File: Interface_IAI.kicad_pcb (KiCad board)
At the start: 2 copper layers, 54 x 63 mm, 20 parts, among them J1 ADWIN_DIO32, J2 ALIM_5V, J3 SCON_PULSE, J4 SCON_FEEDBACK, J5 ADWIN_CO4T, U1 AM26LS31CN, U2 AM26LS32ACN

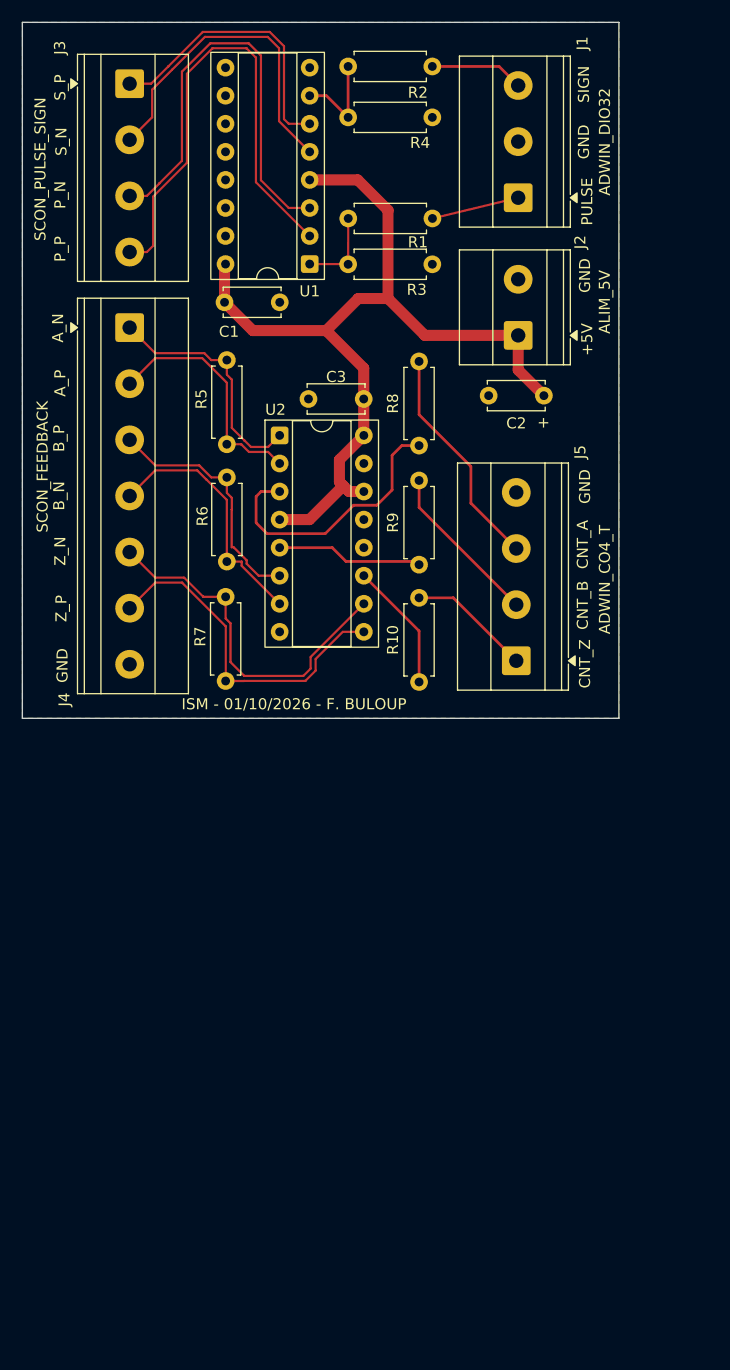
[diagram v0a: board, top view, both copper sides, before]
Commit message: Update board
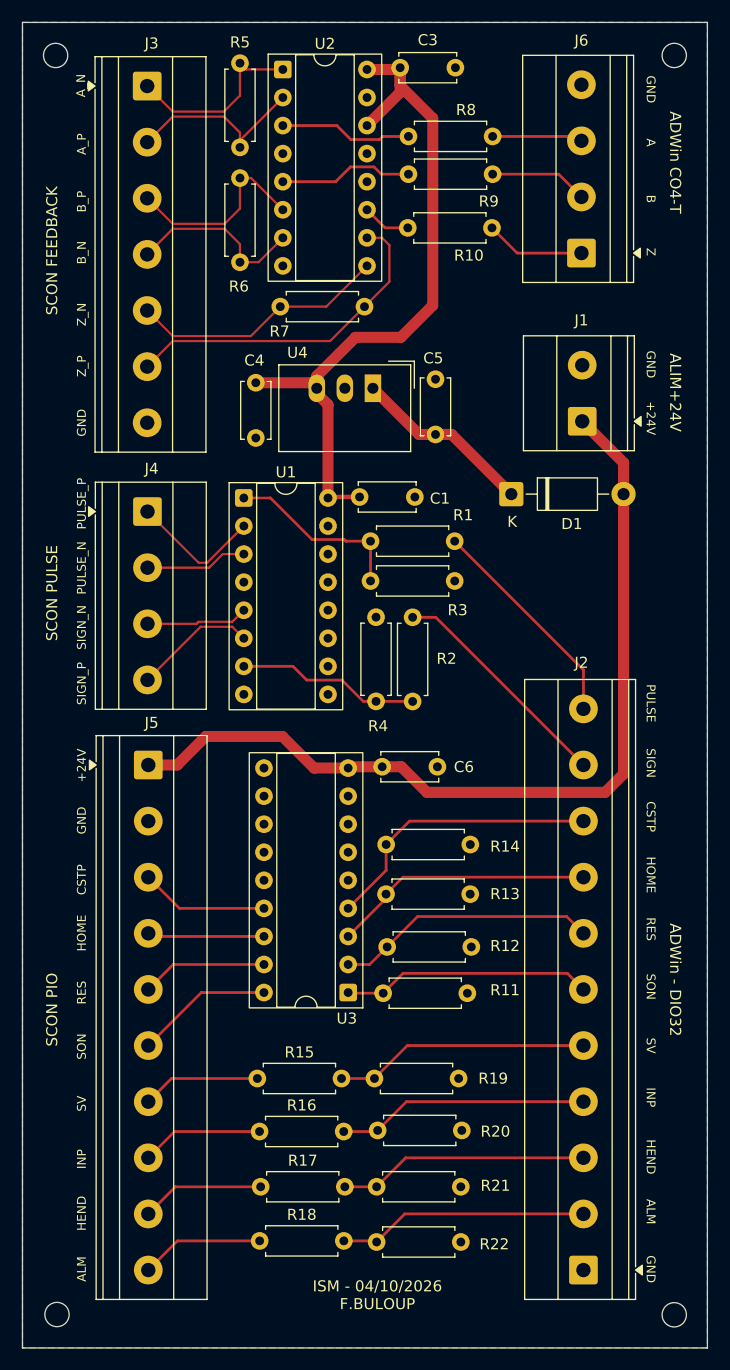
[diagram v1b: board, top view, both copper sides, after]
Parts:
- removed C2: 10uF, Capacitor_THT:C_Disc_D5.0mm_W2.5mm_P5.00mm
- added C4: 10uF, Capacitor_THT:C_Disc_D5.0mm_W2.5mm_P5.00mm, F.Cu at (71.1, 82.6)
- added C5: 10uF 50V, Capacitor_THT:C_Disc_D5.0mm_W2.5mm_P5.00mm, F.Cu at (87.4, 87.3)
- added C6: 100nF, Capacitor_THT:C_Disc_D5.0mm_W2.5mm_P5.00mm, F.Cu at (82.6, 117.4)
- added D1: 1N5819, Diode_THT:D_DO-41_SOD81_P10.16mm_Horizontal, F.Cu at (94.3, 92.7)
- added H1: MountingHole, MountingHole:MountingHole_2.2mm_M2, F.Cu at (109.0, 53.0)
- added H2: MountingHole, MountingHole:MountingHole_2.2mm_M2, F.Cu at (109.0, 167.0)
- added H3: MountingHole, MountingHole:MountingHole_2.2mm_M2, F.Cu at (53.0, 53.0)
- added H4: MountingHole, MountingHole:MountingHole_2.2mm_M2, F.Cu at (53.1, 167.0)
- added J6: ADWin CO4-T, TerminalBlock_Phoenix:TerminalBlock_Phoenix_MKDS-1,5-4-5.08_1x04_P5.08mm_Horizontal, F.Cu at (100.6, 70.9)
- added R11: 10k, Resistor_THT:R_Axial_DIN0207_L6.3mm_D2.5mm_P7.62mm_Horizontal, F.Cu at (82.7, 137.9)
- added R12: 10k, Resistor_THT:R_Axial_DIN0207_L6.3mm_D2.5mm_P7.62mm_Horizontal, F.Cu at (83.0, 133.7)
- added R13: 10k, Resistor_THT:R_Axial_DIN0207_L6.3mm_D2.5mm_P7.62mm_Horizontal, F.Cu at (82.9, 128.9)
- added R14: 10k, Resistor_THT:R_Axial_DIN0207_L6.3mm_D2.5mm_P7.62mm_Horizontal, F.Cu at (82.9, 124.4)
- added R15: 10k, Resistor_THT:R_Axial_DIN0207_L6.3mm_D2.5mm_P7.62mm_Horizontal, F.Cu at (71.3, 145.6)
- added R16: 10k, Resistor_THT:R_Axial_DIN0207_L6.3mm_D2.5mm_P7.62mm_Horizontal, F.Cu at (71.5, 150.4)
- added R17: 10k, Resistor_THT:R_Axial_DIN0207_L6.3mm_D2.5mm_P7.62mm_Horizontal, F.Cu at (71.6, 155.4)
- added R18: 10k, Resistor_THT:R_Axial_DIN0207_L6.3mm_D2.5mm_P7.62mm_Horizontal, F.Cu at (71.5, 160.3)
- added R19: 2.2k, Resistor_THT:R_Axial_DIN0207_L6.3mm_D2.5mm_P7.62mm_Horizontal, F.Cu at (81.9, 145.6)
- added R20: 2.2k, Resistor_THT:R_Axial_DIN0207_L6.3mm_D2.5mm_P7.62mm_Horizontal, F.Cu at (82.2, 150.3)
- added R21: 2.2k, Resistor_THT:R_Axial_DIN0207_L6.3mm_D2.5mm_P7.62mm_Horizontal, F.Cu at (82.1, 155.4)
- added R22: 2.2k, Resistor_THT:R_Axial_DIN0207_L6.3mm_D2.5mm_P7.62mm_Horizontal, F.Cu at (82.1, 160.4)
- added U3: TBD62783APG, Package_DIP:DIP-18_W7.62mm_Socket, F.Cu at (79.5, 137.8)
- added U4: TSR1-2450E, Converter_DCDC:Converter_DCDC_TRACO_TSR-1_THT, F.Cu at (81.7, 83.1)
- J1: value ADWIN_DIO32 -> +24V; footprint TerminalBlock_Phoenix:TerminalBlock_Phoenix_MKDS-1,5-3-5.08_1x03_P5.08mm_Horizontal -> TerminalBlock_Phoenix:TerminalBlock_Phoenix_MKDS-1,5-2-5.08_1x02_P5.08mm_Horizontal
- J2: value ALIM_5V -> ADWIN_DIO32; footprint TerminalBlock_Phoenix:TerminalBlock_Phoenix_MKDS-1,5-2-5.08_1x02_P5.08mm_Horizontal -> TerminalBlock_Phoenix:TerminalBlock_Phoenix_MKDS-1,5-11-5.08_1x11_P5.08mm_Horizontal
- J3: value SCON_PULSE -> SCON_FEEDBACK; footprint TerminalBlock_Phoenix:TerminalBlock_Phoenix_MKDS-1,5-4-5.08_1x04_P5.08mm_Horizontal -> TerminalBlock_Phoenix:TerminalBlock_Phoenix_MKDS-1,5-7-5.08_1x07_P5.08mm_Horizontal
- J4: value SCON_FEEDBACK -> SCON_PULSE; footprint TerminalBlock_Phoenix:TerminalBlock_Phoenix_MKDS-1,5-7-5.08_1x07_P5.08mm_Horizontal -> TerminalBlock_Phoenix:TerminalBlock_Phoenix_MKDS-1,5-4-5.08_1x04_P5.08mm_Horizontal
- J5: value ADWIN_CO4T -> SCON_PIO; footprint TerminalBlock_Phoenix:TerminalBlock_Phoenix_MKDS-1,5-4-5.08_1x04_P5.08mm_Horizontal -> TerminalBlock_Phoenix:TerminalBlock_Phoenix_MKDS-1,5-10-5.08_1x10_P5.08mm_Horizontal
- U1: value AM26LS31CN -> AM26LS31
- U2: value AM26LS32ACN -> AM26LS32
- moved J2 84.8 mm to (100.8, 162.9)
- moved R4 52.9 mm to (82.0, 111.5), turned to 90 degrees
- moved R2 49.9 mm to (85.3, 103.9), turned to -90 degrees
- moved R10 41.1 mm to (84.9, 68.6), turned to 0 degrees
- moved R9 35.4 mm to (84.9, 63.7), turned to 0 degrees
- moved J5 34.6 mm to (61.4, 117.2), turned to -90 degrees
- moved U2 33.1 mm to (73.6, 54.3)
- moved C3 30.2 mm to (84.2, 54.1), turned to 0 degrees
- moved R1 29.3 mm to (89.1, 97.0)
- moved R7 29.1 mm to (81.0, 75.7), turned to 180 degrees
- moved R3 28.7 mm to (81.5, 100.6)
- moved R8 28.0 mm to (84.9, 60.3), turned to 0 degrees
- moved R6 27.1 mm to (69.7, 64.1)
- moved R5 26.9 mm to (69.7, 61.3)
- moved U1 22.0 mm to (70.0, 93.1), turned to 0 degrees
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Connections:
- J1 pad 1: /DIO_PULSE -> +24V
- J2 pad 1: +5V -> GND
- J2 pad 2: GND -> /DIO_ALM
- J3 pad 1: /SIGN_P -> /FB_A_N
- J3 pad 2: /SIGN_N -> /FB_A_P
- J3 pad 3: /PULSE_N -> /FB_B_P
- J3 pad 4: /PULSE_P -> /FB_B_N
- J4 pad 1: /FB_A_N -> /PULSE_P
- J4 pad 2: /FB_A_P -> /PULSE_N
- J4 pad 3: /FB_B_P -> /SIGN_N
- J4 pad 4: /FB_B_N -> /SIGN_P
- J5 pad 1: /CNT_Z -> +24V
- J5 pad 2: /CNT_B -> GND
- J5 pad 3: /CNT_A -> /SCON_CSTP
- J5 pad 4: GND -> /SCON_HOME
- U1 pad 4: +5V -> GND
- U2 pad 4: +5V -> GND
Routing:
- net +24V: track 0.00 -> 80.4 mm
- net /PULSE_P: track 44.9 -> 12.0 mm
- net /PULSE_N: track 39.5 -> 9.23 mm
- net /DIO_CSTP: track 0.00 -> 25.9 mm
- net /DIO_HOME: track 0.00 -> 23.8 mm
- net /DIO_RES: track 0.00 -> 23.7 mm
- net /DIO_SV: track 0.00 -> 23.1 mm
- net /DIO_INP: track 0.00 -> 22.8 mm
- net /DIO_ALM: track 0.00 -> 22.8 mm
- net /DIO_HEND: track 0.00 -> 22.7 mm
- net /DIO_SON: track 0.00 -> 22.7 mm
- net /SIGN_N: track 29.8 -> 9.23 mm
- net /DIO_PULSE: track 0.00 -> 20.0 mm
- net /PULSE_TTL: track 0.00 -> 16.7 mm
- net /VIN_REG: track 0.00 -> 16.5 mm
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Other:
- board size 54 x 63 mm -> 62 x 120 mm
- board text added: "+24V"
- board text added: "A"
- board text added: "ADWin - DIO32"
- board text added: "ADWin CO4-T"
- board text added: "ALIM+24V"
- board text added: "ALM"
- board text added: "B"
- board text added: "CSTP"
- board text added: "HEND"
- board text added: "HOME"
- board text added: "INP"
- board text added: "ISM - 04/10/2026 F.BULOUP"
- board text added: "PULSE_N"
- board text added: "PULSE_P"
- board text added: "RES"
- board text added: "SCON FEEDBACK"
- board text added: "SCON PIO"
- board text added: "SCON PULSE"
- board text added: "SIGN_N"
- board text added: "SIGN_P"
- board text added: "SON"
- board text added: "SV"
- board text added: "Z"
- board text removed: "+"
- board text removed: "+5V"
- board text removed: "ADWIN_CO4_T"
- board text removed: "ADWIN_DIO32"
- board text removed: "ALIM_5V"
- board text removed: "CNT_A"
- board text removed: "CNT_B"
- board text removed: "CNT_Z"
- board text removed: "ISM - 01/10/2026 - F. BULOUP"
- board text removed: "P_N"
- board text removed: "P_P"
- board text removed: "SCON_FEEDBACK"
- board text removed: "SCON_PULSE_SIGN"
- board text removed: "S_N"
- board text removed: "S_P"
